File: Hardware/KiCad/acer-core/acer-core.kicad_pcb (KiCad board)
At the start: 2 copper layers, 35 x 41.8 mm, 26 parts, among them J1 USB_C_Receptacle_USB2.0_16P, J2 Conn_01x10_Pin, J3 Conn_01x10_Pin, J4 Conn_01x16_Socket, Q1 AO3401A, SW1 RESET, SW2 USER, U1 ESP32-S3-WROOM-1, U2 USBLC6-2SC6, U3 WIO-SX1262, U4 TLV75733PDBV

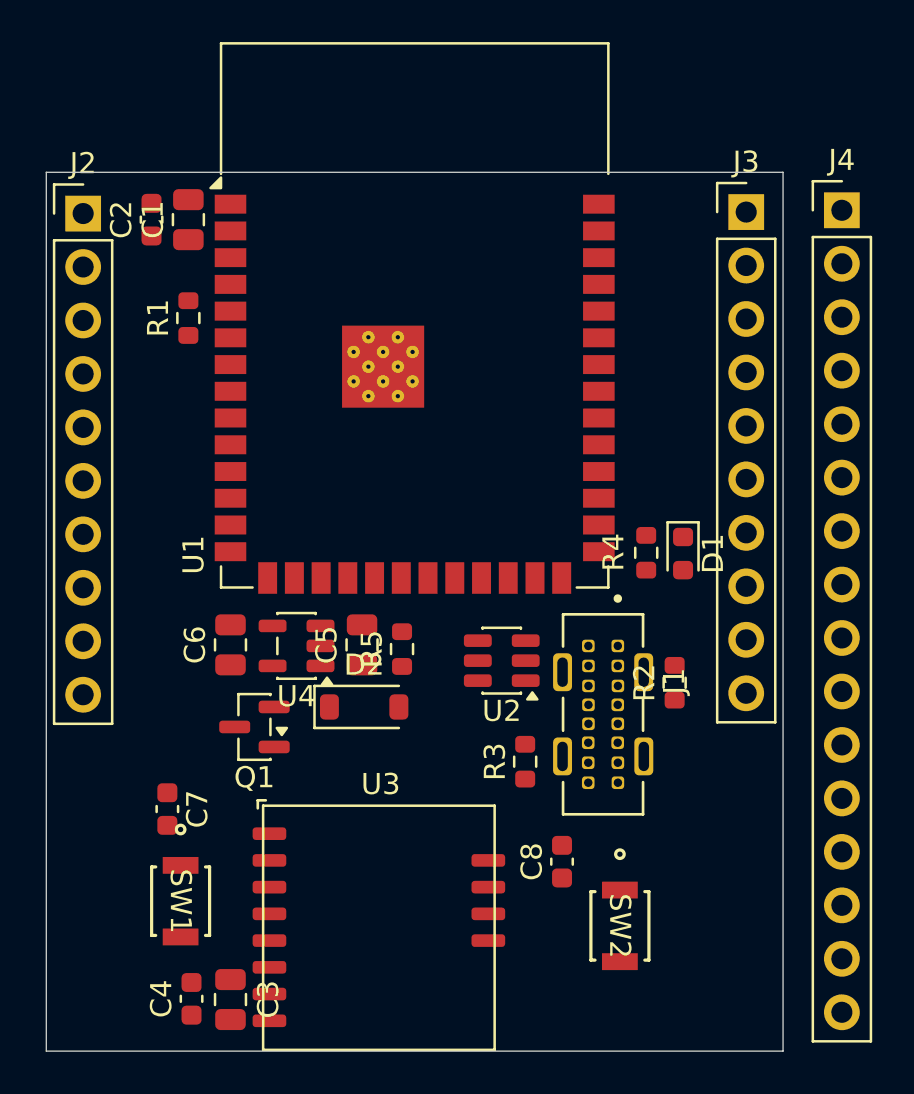
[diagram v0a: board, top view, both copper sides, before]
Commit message: Routing Done
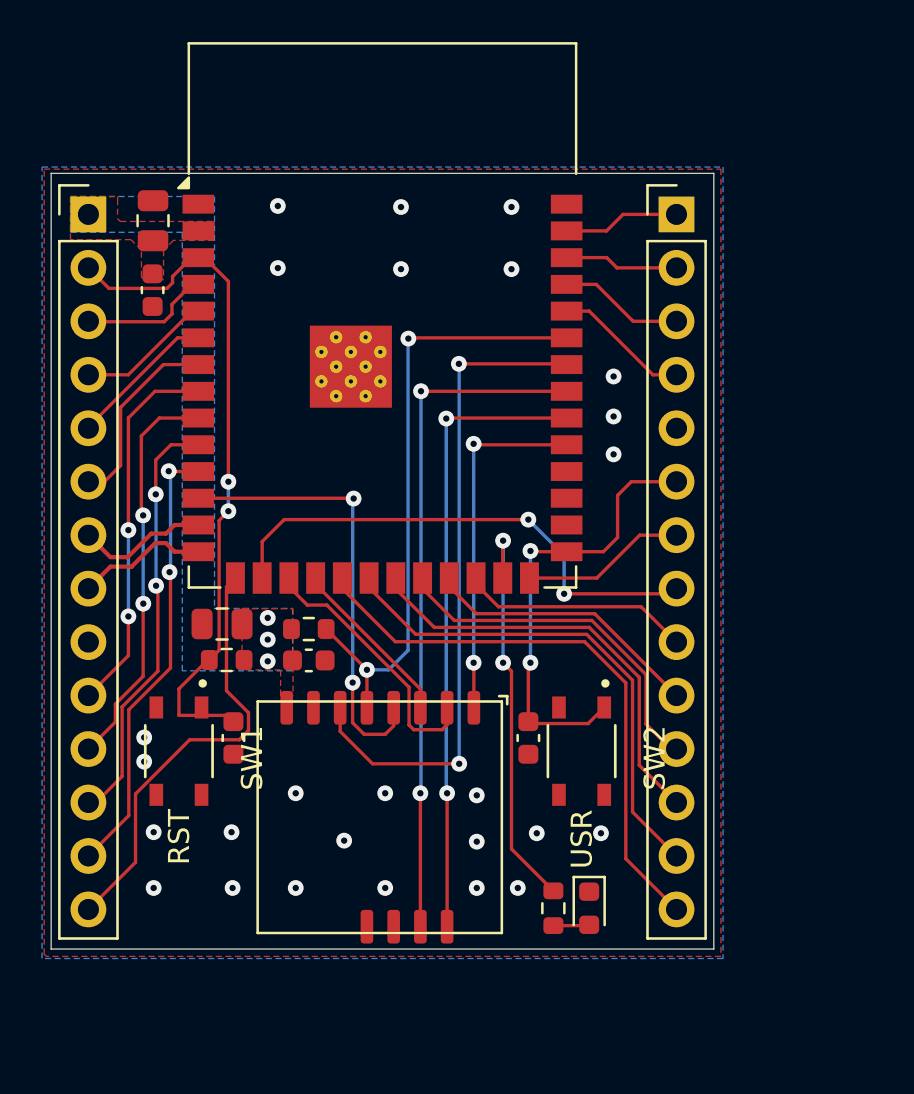
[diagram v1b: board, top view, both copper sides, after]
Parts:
- removed C7, C8: 0.1uF, Capacitor_SMD:C_0603_1608Metric
- removed D2: 1N5817W, Diode_SMD:D_SOD-123
- removed J3: Conn_01x10_Pin, Connector_PinHeader_2.54mm:PinHeader_1x10_P2.54mm_Vertical
- removed J4: Conn_01x16_Socket, Connector_PinHeader_2.54mm:PinHeader_1x16_P2.54mm_Vertical
- removed Q1: AO3401A, Package_TO_SOT_SMD:SOT-23
- removed R4: 330, Resistor_SMD:R_0603_1608Metric
- removed R5: 100K, Resistor_SMD:R_0603_1608Metric
- removed U3: WIO-SX1262, SB-Lib:Wio-SX1262-SB
- removed U4: TLV75733PDBV, Package_TO_SOT_SMD:SOT-23-5
- added G***: LOGO, SB-Logos:EG_Logo_12mm_SilkScreen, B.Cu at (138.5, 94.8)
- added REF**: KiCad-Logo2_5mm_SilkScreen, Symbol:KiCad-Logo2_5mm_SilkScreen, B.Cu at (138.5, 111.6)
- C3, C6: value 10uF -> 0.1uF; footprint Capacitor_SMD:C_0805_2012Metric -> Capacitor_SMD:C_0603_1608Metric
- D1: value Blue 2.9V -> Green 2.1V
- J1: value USB_C_Receptacle_USB2.0_16P -> Conn_01x14_Pin; footprint SB-Lib:CUI_UJ20-C-V-C-3-SMT-TR -> Connector_PinHeader_2.54mm:PinHeader_1x14_P2.54mm_Vertical
- J2: value Conn_01x10_Pin -> Conn_01x14_Pin; footprint Connector_PinHeader_2.54mm:PinHeader_1x10_P2.54mm_Vertical -> Connector_PinHeader_2.54mm:PinHeader_1x14_P2.54mm_Vertical
- R2: value 5K1 -> 130
- R3: value 5K1 -> 10K
- SW1, SW2: footprint SB-Lib:B3U-1000P -> SB_Button_Switch_SMD:SW_SKRPABE010
- U2: value USBLC6-2SC6 -> WIO-SX1262; footprint Package_TO_SOT_SMD:SOT-23-6 -> SB_RF_Module:Wio-SX1262-SB
- moved J1 34.1 mm to (124.5, 81.0), turned to 0 degrees
- moved J2 28.2 mm to (152.4, 81.0)
- moved C4 20.2 mm to (145.4, 105.9), turned to -90 degrees
- moved D1 17.4 mm to (148.3, 114.0)
- moved R1 16.3 mm to (131.1, 102.2), turned to 0 degrees
- moved C3 12.4 mm to (131.4, 105.9), turned to -90 degrees
- moved R2 12.2 mm to (146.6, 114.0)
- moved R3 12.1 mm to (135.0, 100.7), turned to 180 degrees
- moved SW2 8.50 mm to (147.9, 106.5)
- moved SW1 7.13 mm to (128.8, 106.5)
- moved C5 6.72 mm to (130.8, 100.5), turned to 180 degrees
- moved C6 3.79 mm to (135.0, 102.2), turned to 0 degrees
- moved C2 3.35 mm to (127.5, 84.6), turned to -90 degrees
- moved U2 1.94 mm to (144.1, 104.1)
- moved C1 1.68 mm to (127.6, 81.3)
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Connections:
- C3 pad 1: +3.3V -> /EN
- C4 pad 1: +3.3V -> /USER
- C5 pad 1: Net-(D2-K) -> +3.3V
- J2 pad 1: +3.3V -> /IO1
- J2 pad 10: /IO12 -> /IO21
- J2 pad 2: +5V -> /IO2
- J2 pad 3: /IO18 -> /TXD0
- J2 pad 4: /IO17 -> /RXD0
- J2 pad 6: /IO16 -> /USER
- J2 pad 7: /IO15 -> /IO45
- J2 pad 8: /IO14 -> /IO46
- J2 pad 9: /IO13 -> /IO47
- R2 pad 1: Net-(J1-CC1) -> Net-(D1-A)
- R2 pad 2: GND -> Net-(U1-IO48)
- R3 pad 1: Net-(J1-CC2) -> /LORA_RST
- R3 pad 2: GND -> +3.3V
- U1 pad 16: unconnected-(U1-IO46-Pad16) -> /IO46
- U1 pad 19: unconnected-(U1-IO11-Pad19) -> /IO11
- U1 pad 23: unconnected-(U1-IO21-Pad23) -> /IO21
- U1 pad 24: unconnected-(U1-IO47-Pad24) -> /IO47
- U1 pad 26: unconnected-(U1-IO45-Pad26) -> /IO45
- U1 pad 6: unconnected-(U1-IO6-Pad6) -> /IO6
- U1 pad 7: unconnected-(U1-IO7-Pad7) -> /IO7
- U2 pad 1: Net-(J1-D--PadA7) -> /LORA_RF_SW1
- U2 pad 2: GND -> /LORA_MISO
- U2 pad 3: Net-(J1-D+-PadA6) -> /LORA_MOSI
- U2 pad 4: /USB_D+ -> /LORA_SCK
- U2 pad 5: Vbus -> /LORA_RST
- U2 pad 6: /USB_D- -> /LORA_NSS
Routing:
- net /EN: track 0.00 -> 32.6 mm, vias 0 -> 2
- net /LORA_BUSY: track 0.00 -> 32.4 mm, vias 0 -> 2
- net /LORA_NSS: track 0.00 -> 31.6 mm, vias 0 -> 2
- net /LORA_DIO: track 0.00 -> 29.9 mm, vias 0 -> 2
- net /LORA_RST: track 0.00 -> 29.2 mm, vias 0 -> 2
- net /IO11: track 0.00 -> 27.6 mm
- net /IO46: track 0.00 -> 24.5 mm, vias 0 -> 2
- net /IO12: track 0.00 -> 24.0 mm
- net /USER: track 0.00 -> 22.0 mm, vias 0 -> 2
- net /IO18: track 0.00 -> 21.4 mm, vias 0 -> 2
- net /LORA_SCK: track 0.00 -> 21.3 mm, vias 0 -> 2
- net /IO3: track 0.00 -> 20.9 mm
- net /IO13: track 0.00 -> 20.5 mm
- net /IO17: track 0.00 -> 20.2 mm, vias 0 -> 2
- net Net-(U1-IO48): track 0.00 -> 19.4 mm, vias 0 -> 2
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- added copper zone on B.Cu, net +3.3V
- added copper zone on F.Cu, net +3.3V
- added copper zone on B.Cu, net GND
- added copper zone on F.Cu, net GND
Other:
- board size 35 x 41.8 mm -> 31.5 x 36.9 mm
- board text added: "3.3V"
- board text added: "EN"
- board text added: "GND"
- board text added: "IO1"
- board text added: "IO11"
- board text added: "IO12"
- board text added: "IO13"
- board text added: "IO14"
- board text added: "IO15"
- board text added: "IO16"
- board text added: "IO17"
- board text added: "IO18"
- board text added: "IO2"
- board text added: "IO21"
- board text added: "IO3"
- board text added: "IO4"
- board text added: "IO45"
- board text added: "IO46"
- board text added: "IO47"
- board text added: "IO5"
- board text added: "IO6"
- board text added: "IO7"
- board text added: "RST"
- board text added: "RXD0"
- board text added: "TXD0"
- board text added: "USB+"
- board text added: "USB-"
- board text added: "USER"
- board text added: "USR"
